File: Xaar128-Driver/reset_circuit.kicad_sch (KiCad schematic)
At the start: 43 parts, among them Q1 DMN2075U, Q2 DMN2075U, Q3 DMN2075U, Q7 DMG2305UX, U1 6N135, U2 6N135, U3 74HC173

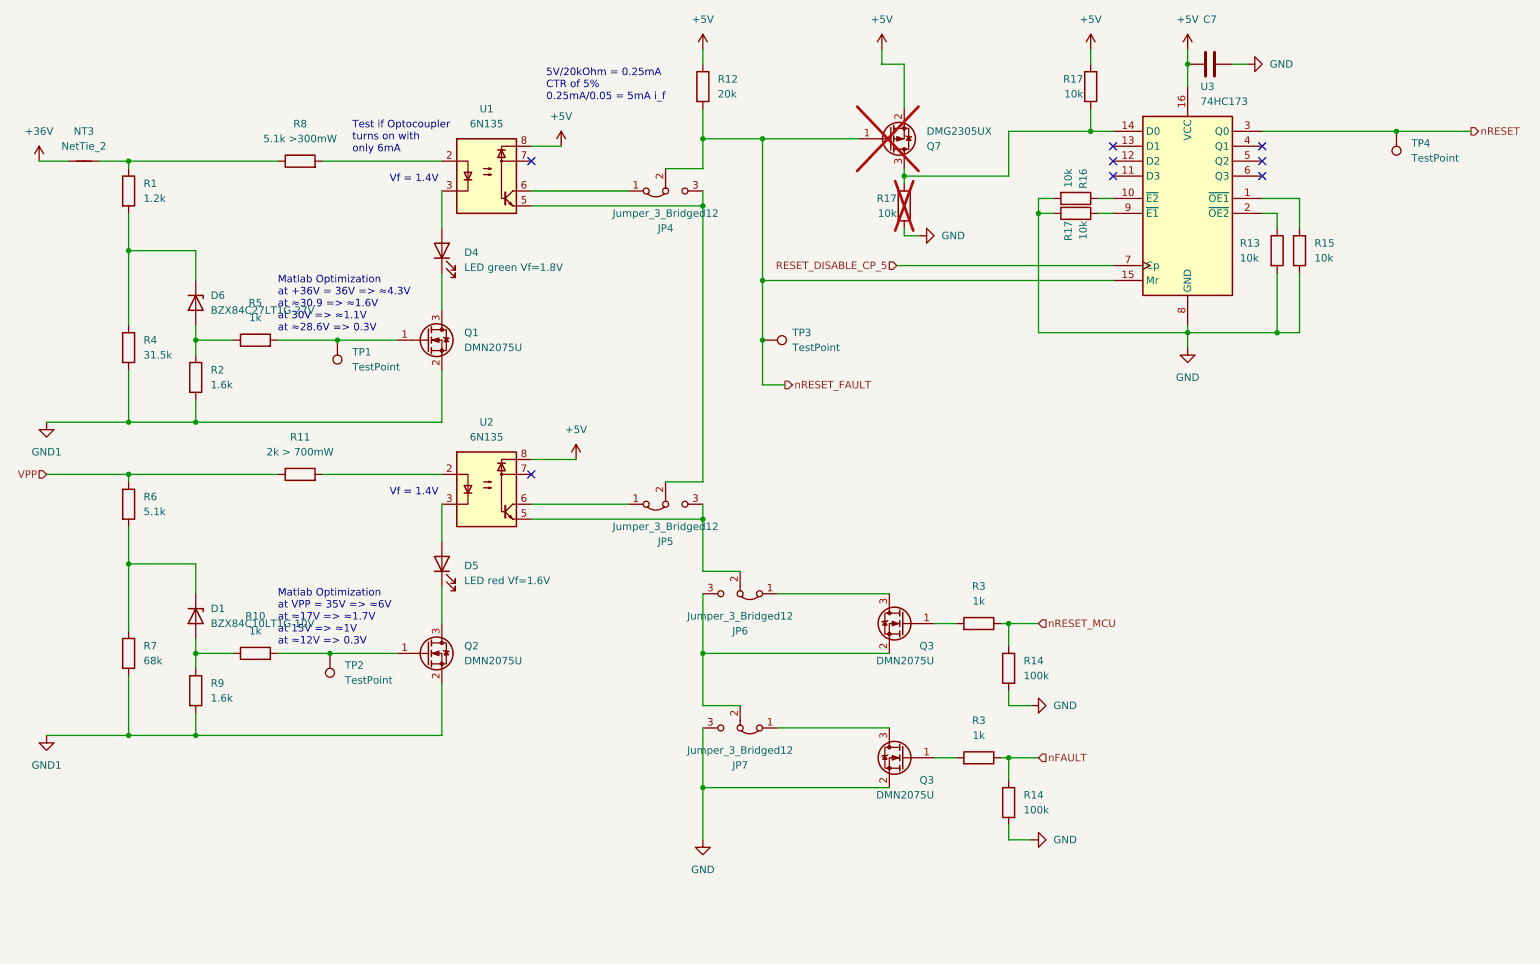
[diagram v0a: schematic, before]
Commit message: more routing
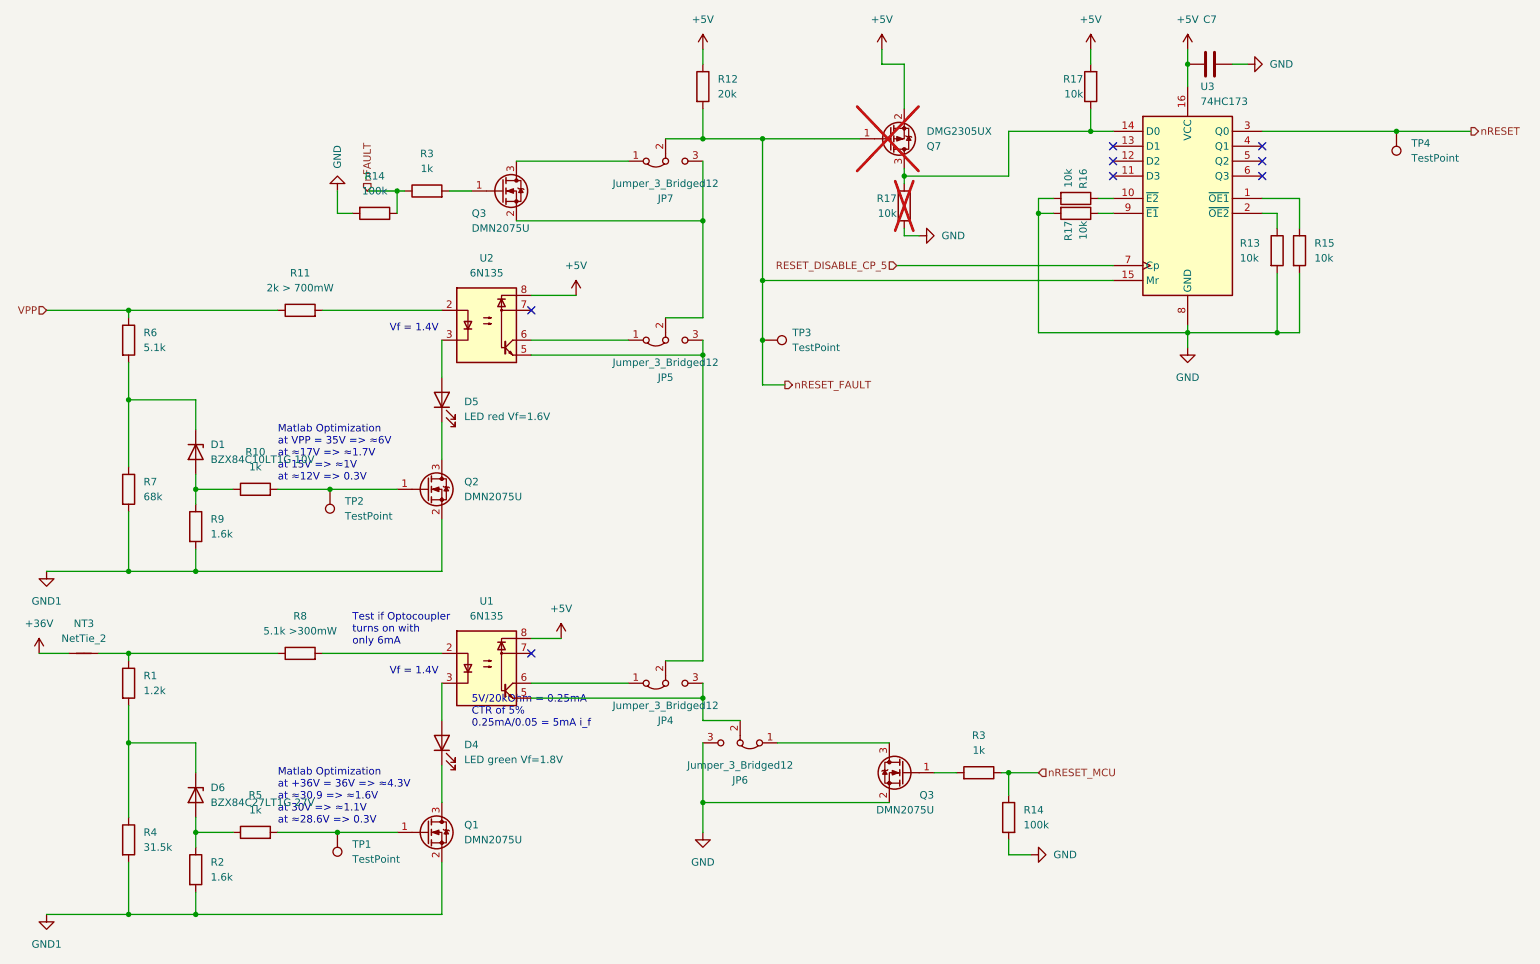
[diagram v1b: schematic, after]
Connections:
- net GND: now also JP6.3 (B), Q3.2 (S); no longer JP7.3 (B), Q3.2 (S)
- net nRESET_FAULT: now also JP7.2 (C); no longer JP4.2 (C)
- net at JP5.3 (B), U2.5: now also JP4.2 (C); no longer JP6.2 (C)
- net at JP4.3 (B), U1.5: now also JP6.2 (C); no longer JP5.2 (C)
- new net: JP5.2 (C), JP7.3 (B), Q3.2 (S)
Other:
- moved on the sheet: D1, D4, D5, D6, JP4, JP5, JP6, NT3, Q1, Q2, Q3, R1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
